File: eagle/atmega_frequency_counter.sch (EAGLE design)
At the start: 49 parts, among them IC1 TL071P, IC2 TL072P, T1 2N3904, U1 ATMEGA328P_PDIP

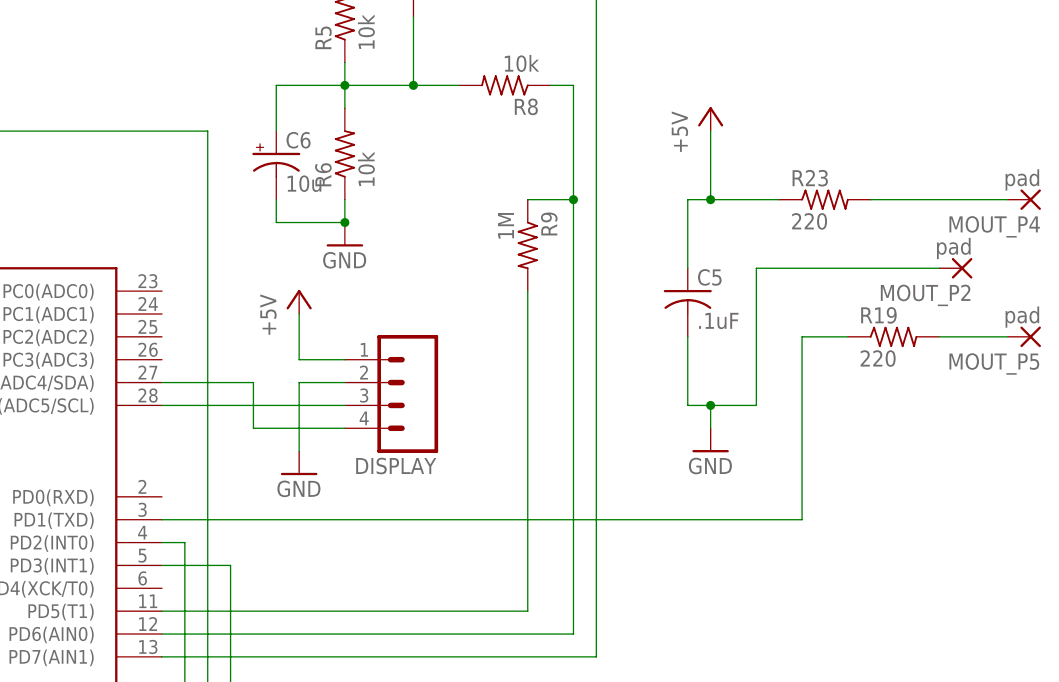
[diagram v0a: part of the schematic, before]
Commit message: layout
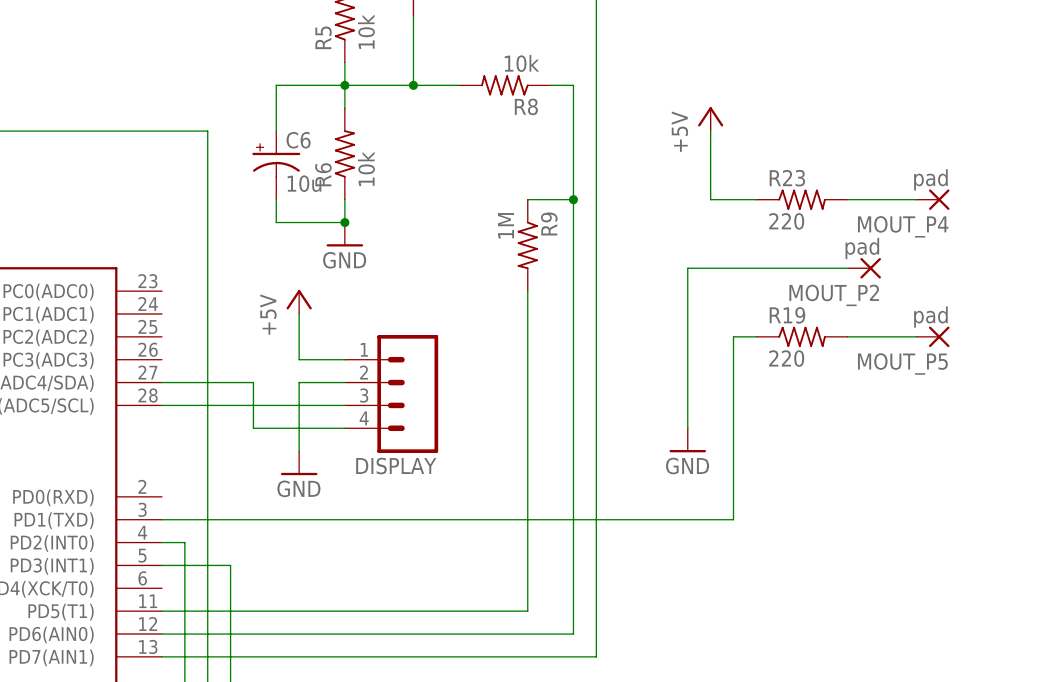
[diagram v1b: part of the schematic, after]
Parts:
- removed C5: .1uF, rcl:C-US050-024X044
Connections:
- net +5V: no longer C5.1
- net GND: no longer C5.2
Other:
- moved on the sheet: MOUT_P2, MOUT_P4, MOUT_P5, R19, R23
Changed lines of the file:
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@@
 <grid distance="0.1" unitdist="inch" unit="inch" style="lines" multiple="1" display="no" altdistance="0.01" altunitdist="inch" altunit="inch"/>
 <layers>
-<layer number="1" name="Top" color="4" fill="1" visible="yes" active="no"/>
-<layer number="16" name="Bottom" color="1" fill="1" visible="yes" active="no"/>
-<layer number="17" name="Pads" color="2" fill="1" visible="yes" active="no"/>
-<layer number="18" name="Vias" color="2" fill="1" visible="yes" active="no"/>
-<layer number="19" name="Unrouted" color="6" fill="1" visible="yes" active="no"/>
-<layer number="20" name="Dimension" color="15" fill="1" visible="yes" active="no"/>
-<layer number="21" name="tPlace" color="7" fill="1" visible="yes" active="no"/>
-<layer number="22" name="bPlace" color="7" fill="1" visible="yes" active="no"/>
-<layer number="23" name="tOrigins" color="15" fill="1" visible="yes" active="no"/>
-<layer number="24" name="bOrigins" color="15" fill="1" visible="yes" active="no"/>
-<layer number="25" name="tNames" color="7" fill="1" visible="yes" active="no"/>
-<layer number="26" name="bNames" color="7" fill="1" visible="yes" active="no"/>
-<layer number="27" name="tValues" color="7" fill="1" visible="yes" active="no"/>
-<layer number="28" name="bValues" color="7" fill="1" visible="yes" active="no"/>
+<layer number="1" name="Top" color="4" fill="1" visible="no" active="no"/>
+<layer number="16" name="Bottom" color="1" fill="1" visible="no" active="no"/>
+<layer number="17" name="Pads" color="2" fill="1" visible="no" active="no"/>
+<layer number="18" name="Vias" color="2" fill="1" visible="no" active="no"/>
+<layer number="19" name="Unrouted" color="6" fill="1" visible="no" active="no"/>
+<layer number="20" name="Dimension" color="15" fill="1" visible="no" active="no"/>
+<layer number="21" name="tPlace" color="7" fill="1" visible="no" active="no"/>
+<layer number="22" name="bPlace" color="7" fill="1" visible="no" active="no"/>
+<layer number="23" name="tOrigins" color="15" fill="1" visible="no" active="no"/>
+<layer number="24" name="bOrigins" color="15" fill="1" visible="no" active="no"/>
+<layer number="25" name="tNames" color="7" fill="1" visible="no" active="no"/>
+<layer number="26" name="bNames" color="7" fill="1" visible="no" active="no"/>
+<layer number="27" name="tValues" color="7" fill="1" visible="no" active="no"/>
+<layer number="28" name="bValues" color="7" fill="1" visible="no" active="no"/>
 <layer number="29" name="tStop" color="7" fill="3" visible="no" active="no"/>
 <layer number="30" name="bStop" color="7" fill="6" visible="no" active="no"/>
@@
 <layer number="35" name="tGlue" color="7" fill="4" visible="no" active="no"/>
 <layer number="36" name="bGlue" color="7" fill="5" visible="no" active="no"/>
-<layer number="37" name="tTest" color="7" fill="1" visible="yes" active="no"/>
-<layer number="38" name="bTest" color="7" fill="1" visible="yes" active="no"/>
+<layer number="37" name="tTest" color="7" fill="1" visible="no" active="no"/>
+<layer number="38" name="bTest" color="7" fill="1" visible="no" active="no"/>
 <layer number="39" name="tKeepout" color="4" fill="11" visible="no" active="no"/>
 <layer number="40" name="bKeepout" color="1" fill="11" visible="no" active="no"/>
@@
 <layer number="44" name="Drills" color="7" fill="1" visible="no" active="no"/>
 <layer number="45" name="Holes" color="7" fill="1" visible="no" active="no"/>
-<layer number="46" name="Milling" color="3" fill="1" visible="yes" active="no"/>
-<layer number="47" name="Measures" color="7" fill="1" visible="yes" active="no"/>
-<layer number="48" name="Document" color="7" fill="1" visible="yes" active="no"/>
-<layer number="49" name="Reference" color="7" fill="1" visible="yes" active="no"/>
-<layer number="50" name="dxf" color="7" fill="1" visible="yes" active="no"/>
-<layer number="51" name="tDocu" color="7" fill="1" visible="yes" active="no"/>
-<layer number="52" name="bDocu" color="7" fill="1" visible="yes" active="no"/>
-<layer number="53" name="tGND_GNDA" color="7" fill="9" visible="yes" active="no"/>
-<layer number="54" name="bGND_GNDA" color="1" fill="9" visible="yes" active="no"/>
-<layer number="56" name="wert" color="7" fill="1" visible="yes" active="no"/>
-<layer number="57" name="tCAD" color="7" fill="1" visible="yes" active="no"/>
+<layer number="46" name="Milling" color="3" fill="1" visible="no" active="no"/>
+<layer number="47" name="Measures" color="7" fill="1" visible="no" active="no"/>
+<layer number="48" name="Document" color="7" fill="1" visible="no" active="no"/>
+<layer number="49" name="Reference" color="7" fill="1" visible="no" active="no"/>
+<layer number="50" name="dxf" color="7" fill="1" visible="no" active="no"/>
+<layer number="51" name="tDocu" color="7" fill="1" visible="no" active="no"/>
+<layer number="52" name="bDocu" color="7" fill="1" visible="no" active="no"/>
+<layer number="53" name="tGND_GNDA" color="7" fill="9" visible="no" active="no"/>
+<layer number="54" name="bGND_GNDA" color="1" fill="9" visible="no" active="no"/>
+<layer number="56" name="wert" color="7" fill="1" visible="no" active="no"/>
+<layer number="57" name="tCAD" color="7" fill="1" visible="no" active="no"/>
 <layer number="90" name="Modules" color="5" fill="1" visible="yes" active="yes"/>
 <layer number="91" name="Nets" color="2" fill="1" visible="yes" active="yes"/>
@@
 <part name="P+3" library="supply1" deviceset="+5V" device=""/>
 <part name="GND2" library="supply1" deviceset="GND" device=""/>
-<part name="C5" library="rcl" deviceset="C-US" device="050-024X044" value=".1uF"/>
 <part name="P+14" library="supply1" deviceset="+5V" device=""/>
 <part name="GND17" library="supply1" deviceset="GND" device=""/>
@@
 <instance part="P+3" gate="1" x="58.42" y="73.66"/>
 <instance part="GND2" gate="1" x="58.42" y="53.34"/>
-<instance part="C5" gate="G$1" x="101.6" y="73.66"/>
 <instance part="P+14" gate="1" x="104.14" y="93.98"/>
-<instance part="GND17" gate="1" x="104.14" y="55.88"/>
-<instance part="R19" gate="G$1" x="124.46" y="68.58"/>
-<instance part="MOUT_P5" gate="1" x="139.7" y="68.58" rot="R180"/>
-<instance part="MOUT_P4" gate="1" x="139.7" y="83.82" rot="R180"/>
-<instance part="MOUT_P2" gate="1" x="132.08" y="76.2" rot="R180"/>
-<instance part="R23" gate="G$1" x="116.84" y="83.82"/>
+<instance part="GND17" gate="1" x="101.6" y="55.88"/>
+<instance part="R19" gate="G$1" x="114.3" y="68.58"/>
+<instance part="MOUT_P5" gate="1" x="129.54" y="68.58" rot="R180"/>
+<instance part="MOUT_P4" gate="1" x="129.54" y="83.82" rot="R180"/>
+<instance part="MOUT_P2" gate="1" x="121.92" y="76.2" rot="R180"/>
+<instance part="R23" gate="G$1" x="114.3" y="83.82"/>
 <instance part="T1" gate="G1" x="68.58" y="-17.78"/>
 <instance part="R2" gate="G$1" x="71.12" y="0" rot="R90"/>
@@
 <pinref part="P+14" gate="1" pin="+5V"/>
 <wire x1="104.14" y1="91.44" x2="104.14" y2="83.82" width="0.1524" layer="91"/>
-<pinref part="C5" gate="G$1" pin="1"/>
-<wire x1="101.6" y1="76.2" x2="101.6" y2="83.82" width="0.1524" layer="91"/>
-<wire x1="101.6" y1="83.82" x2="104.14" y2="83.82" width="0.1524" layer="91"/>
-<junction x="104.14" y="83.82"/>
-<wire x1="111.76" y1="83.82" x2="104.14" y2="83.82" width="0.1524" layer="91"/>
+<wire x1="109.22" y1="83.82" x2="104.14" y2="83.82" width="0.1524" layer="91"/>
 <pinref part="R23" gate="G$1" pin="1"/>
 </segment>
@@
 <segment>
 <pinref part="GND17" gate="1" pin="GND"/>
-<wire x1="104.14" y1="58.42" x2="104.14" y2="60.96" width="0.1524" layer="91"/>
-<pinref part="C5" gate="G$1" pin="2"/>
-<wire x1="101.6" y1="68.58" x2="101.6" y2="60.96" width="0.1524" layer="91"/>
-<wire x1="101.6" y1="60.96" x2="104.14" y2="60.96" width="0.1524" layer="91"/>
-<junction x="104.14" y="60.96"/>
 <pinref part="MOUT_P2" gate="1" pin="P"/>
-<wire x1="129.54" y1="76.2" x2="109.22" y2="76.2" width="0.1524" layer="91"/>
-<wire x1="109.22" y1="76.2" x2="109.22" y2="60.96" width="0.1524" layer="91"/>
-<wire x1="109.22" y1="60.96" x2="104.14" y2="60.96" width="0.1524" layer="91"/>
+<wire x1="119.38" y1="76.2" x2="101.6" y2="76.2" width="0.1524" layer="91"/>
+<wire x1="101.6" y1="76.2" x2="101.6" y2="58.42" width="0.1524" layer="91"/>
 </segment>
 <segment>
@@
 <pinref part="R19" gate="G$1" pin="2"/>
 <pinref part="MOUT_P5" gate="1" pin="P"/>
-<wire x1="137.16" y1="68.58" x2="129.54" y2="68.58" width="0.1524" layer="91"/>
+<wire x1="127" y1="68.58" x2="119.38" y2="68.58" width="0.1524" layer="91"/>
 </segment>
 </net>
@@
 <pinref part="R23" gate="G$1" pin="2"/>
 <pinref part="MOUT_P4" gate="1" pin="P"/>
-<wire x1="121.92" y1="83.82" x2="137.16" y2="83.82" width="0.1524" layer="91"/>
+<wire x1="119.38" y1="83.82" x2="127" y2="83.82" width="0.1524" layer="91"/>
 </segment>
 </net>
@@
 <segment>
 <pinref part="R19" gate="G$1" pin="1"/>
-<wire x1="119.38" y1="68.58" x2="114.3" y2="68.58" width="0.1524" layer="91"/>
-<wire x1="114.3" y1="68.58" x2="114.3" y2="48.26" width="0.1524" layer="91"/>
+<wire x1="109.22" y1="68.58" x2="106.68" y2="68.58" width="0.1524" layer="91"/>
+<wire x1="106.68" y1="68.58" x2="106.68" y2="48.26" width="0.1524" layer="91"/>
 <pinref part="U1" gate="G$1" pin="PD1(TXD)"/>
-<wire x1="114.3" y1="48.26" x2="43.18" y2="48.26" width="0.1524" layer="91"/>
-</segment>
-</net>
+<wire x1="106.68" y1="48.26" x2="43.18" y2="48.26" width="0.1524" layer="91"/>
+</segment>
+</net>
